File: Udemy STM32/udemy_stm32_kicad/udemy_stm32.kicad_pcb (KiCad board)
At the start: 2 copper layers, 28 parts, among them J1 Conn_01x04_Pin, J2 Conn_01x04_Pin, J3 Conn_01x04_Pin, J4 USB_B_Micro, SW1 SW_SPDT, U1 AMS1117-3.3, U2 STM32F103C8T6, Y1 16MHz

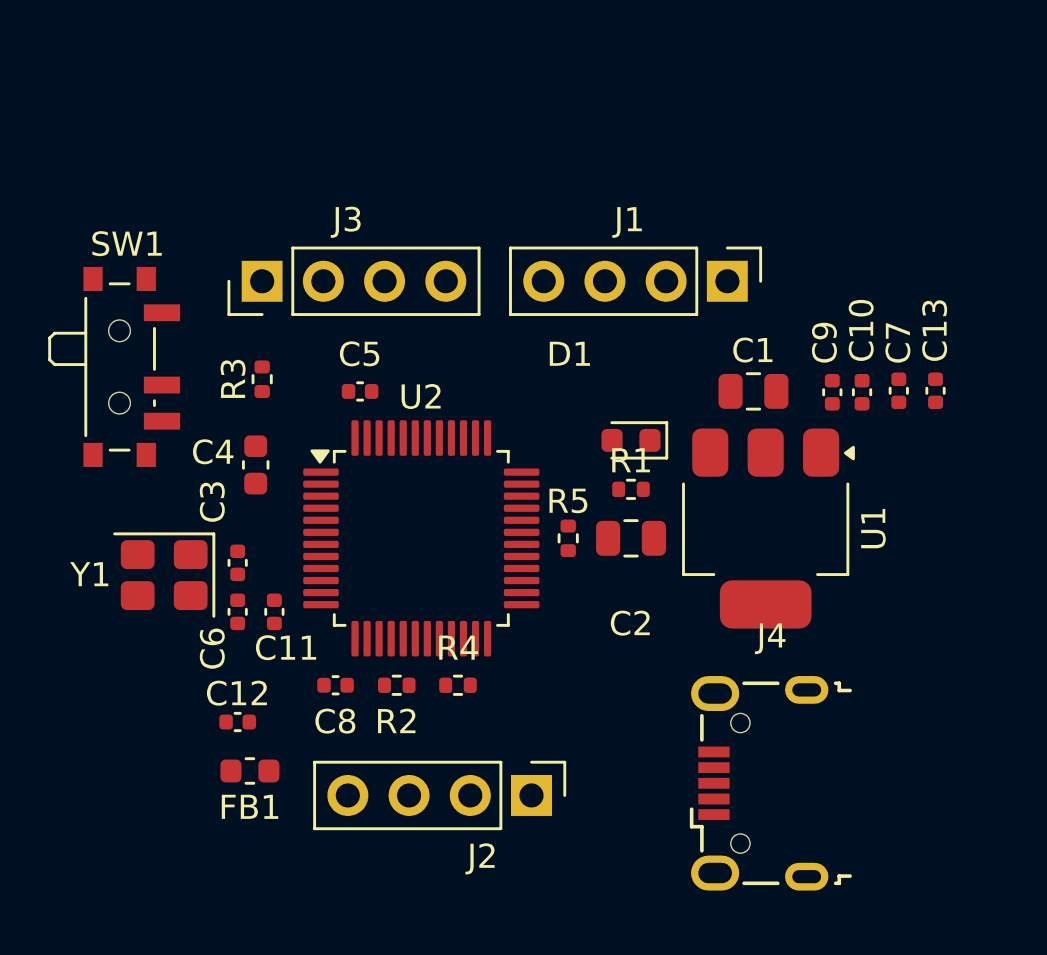
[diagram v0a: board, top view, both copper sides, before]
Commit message: Tinkering around for good placements
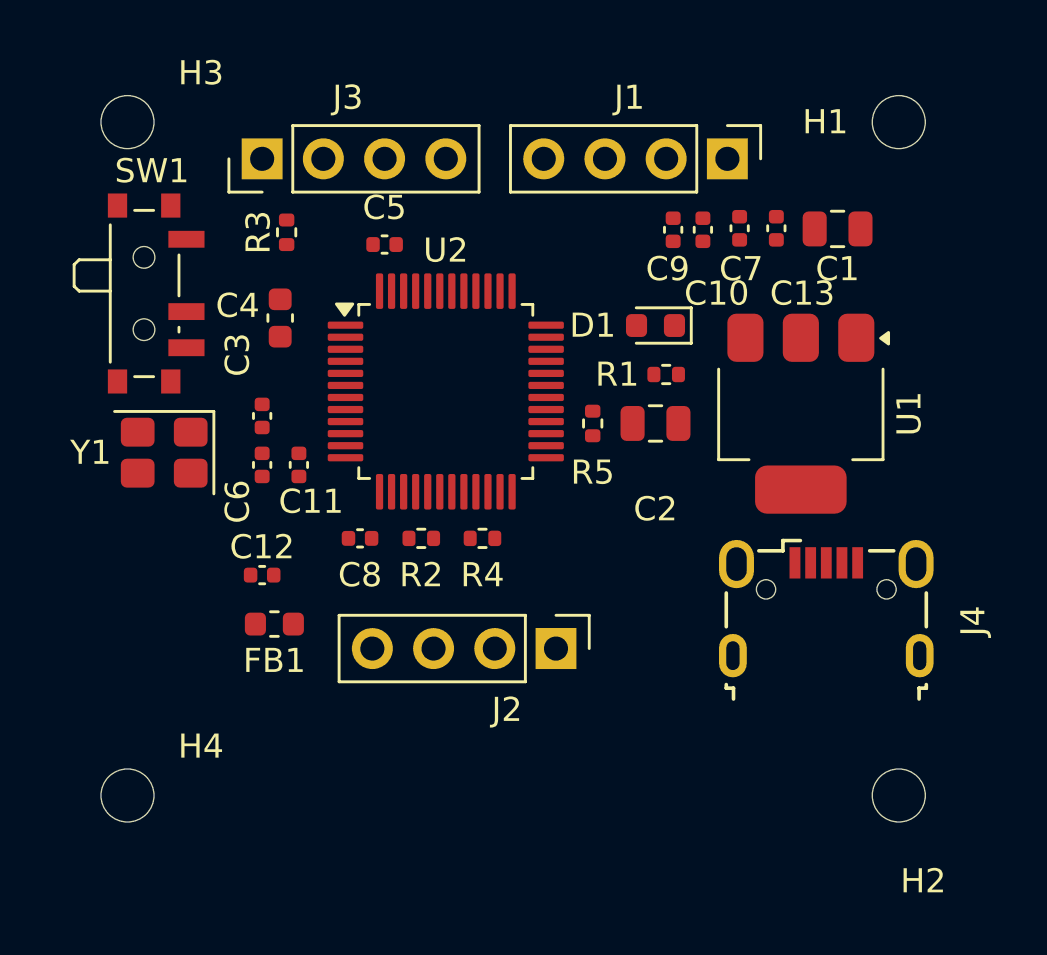
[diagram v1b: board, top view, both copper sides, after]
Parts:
- added H1: MountingHole, MountingHole:MountingHole_2.2mm_M2, F.Cu at (130.0, 71.6)
- added H2: MountingHole, MountingHole:MountingHole_2.2mm_M2, F.Cu at (130.0, 99.6)
- added H3: MountingHole, MountingHole:MountingHole_2.2mm_M2, F.Cu at (98.0, 71.6)
- added H4: MountingHole, MountingHole:MountingHole_2.2mm_M2, F.Cu at (98.0, 99.6)
- moved C10 9.44 mm to (121.9, 76.1)
- moved C9 9.44 mm to (120.7, 76.1)
- moved C13 9.44 mm to (125.0, 76.0)
- moved C7 9.44 mm to (123.4, 76.0)
- moved J4 7.76 mm to (127.0, 91.8), turned to 0 degrees
- moved C1 7.59 mm to (127.5, 76.1)
- moved C3 6.18 mm to (103.6, 83.8)
- moved C4 6.18 mm to (104.4, 79.8)
- moved C5 6.18 mm to (108.7, 76.7)
- moved FB1 6.18 mm to (104.1, 92.5)
- moved J2 6.18 mm to (115.8, 93.5)
- moved R3 6.18 mm to (104.6, 76.2)
- moved U2 6.18 mm to (111.3, 82.8)
- moved C11 6.18 mm to (105.2, 85.9)
- moved C12 6.18 mm to (103.6, 90.4)
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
